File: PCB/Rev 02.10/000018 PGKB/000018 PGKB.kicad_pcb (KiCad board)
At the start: 4 copper layers, 93.5 x 72.5 mm, 156 parts, among them J1 USB C, J2 S4B-PH-SM4-TB, U1 SN74HCS365PWR, U2 SN74HCS365PWR, U3 SN74HCS365PWR, U4 W25Q80DVSSIG, U5 RP2040, U6 MCP1825T-3302E/DC, U7 CAT811TTBI-GT3, Y1 12 MHz

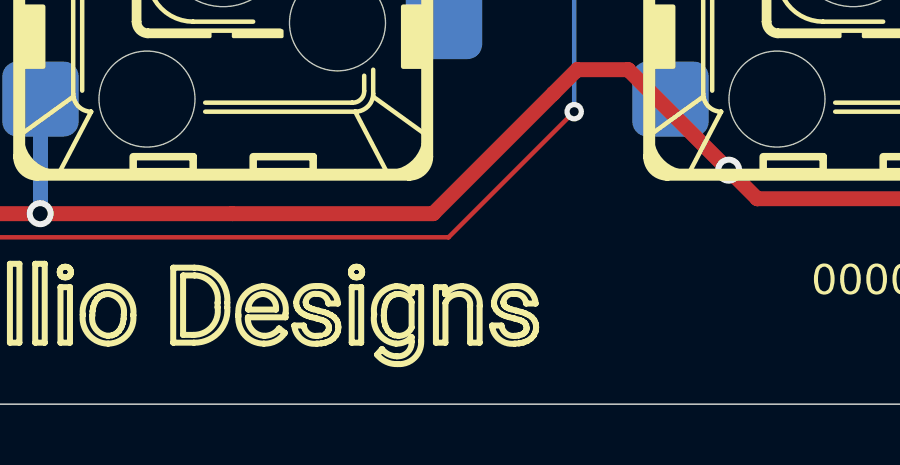
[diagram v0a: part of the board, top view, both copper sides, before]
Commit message: Signals renamed
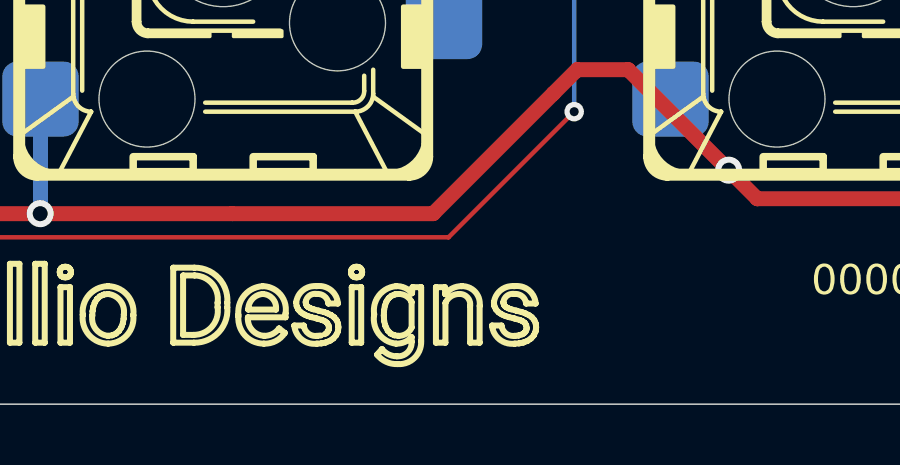
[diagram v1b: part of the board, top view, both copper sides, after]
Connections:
- net /Main/Microcontroller/GPIO12 renamed /Main/Microcontroller/GPIO29
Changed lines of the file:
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@@
 	(net 39 "unconnected-(J1-SBU2-PadB8)")
 	(net 40 "/Main/Microcontroller/NEOPIX_DRIVE")
-	(net 41 "/Main/Microcontroller/GPIO12")
+	(net 41 "/Main/Microcontroller/GPIO29")
 	(net 42 "/Main/Buttons/Button6")
 	(net 43 "/Main/Buttons/Button7")
@@
 		(fp_arc
 			(start 1.31605 -0.683114)
-			(mid 1.907695 -0.405492)
+			(mid 1.907699 -0.405492)
 			(end 2.078018 0.225468)
 			(stroke
@@
 		(fp_arc
 			(start 1.372869 0.972724)
-			(mid 0.966366 0.781547)
+			(mid 0.966362 0.781547)
 			(end 0.82295 0.35584)
 			(stroke
@@
 		(fp_arc
 			(start 3.12764 1.232463)
-			(mid 2.61934 1.092397)
+			(mid 2.619347 1.092399)
 			(end 2.369218 0.628268)
 			(stroke
@@
 		(fp_arc
 			(start 5.03409 0.259459)
-			(mid 5.191951 -0.372877)
+			(mid 5.19195 -0.37288)
 			(end 5.765118 -0.683118)
 			(stroke
@@
 		(fp_arc
 			(start 6.280538 1.013814)
-			(mid 6.045436 1.181019)
+			(mid 6.045436 1.181008)
 			(end 5.761568 1.232468)
 			(stroke
@@
 		(fp_arc
 			(start 7.407765 -0.124568)
-			(mid 7.589655 -0.340729)
+			(mid 7.589656 -0.340694)
 			(end 7.859781 -0.423381)
 			(stroke
@@
 		(fp_arc
 			(start 7.955657 -0.683113)
-			(mid 8.404805 -0.489301)
+			(mid 8.404847 -0.489303)
 			(end 8.54819 -0.02159)
 			(stroke
@@
 		(fp_arc
 			(start 9.708398 -0.423378)
-			(mid 9.968762 -0.344292)
+			(mid 9.96879 -0.344297)
 			(end 10.097 -0.104281)
 			(stroke
@@
 		(fp_arc
 			(start 9.71855 1.232464)
-			(mid 9.210242 1.092402)
+			(mid 9.21027 1.092398)
 			(end 8.960131 0.628268)
 			(stroke
@@
 			(layers "B.Cu" "B.Paste" "B.Mask")
 			(roundrect_rratio 0.25)
-			(net 41 "/Main/Microcontroller/GPIO12")
+			(net 41 "/Main/Microcontroller/GPIO29")
 			(pinfunction "O2")
 			(pintype "tri_state")
@@
 			(layers "B.Cu" "B.Paste" "B.Mask")
 			(roundrect_rratio 0.25)
-			(net 41 "/Main/Microcontroller/GPIO12")
+			(net 41 "/Main/Microcontroller/GPIO29")
 			(pinfunction "GPIO29_ADC3")
 			(pintype "bidirectional")
